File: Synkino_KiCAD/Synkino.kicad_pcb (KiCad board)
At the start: 2 copper layers, 88.4 x 82.3 mm, 180 parts, among them J1 Conn_01x02_Male, J10 EYE8_OUT, J11 EYE4_OUT, J12 2.5mm, J13 EYE5_OUT, J2 2.5mm, J3 3.5mm, J4 Micro_SD_Card_Det_Hirose_DM3AT, J5 EYE1_OUT, J6 EYE6_OUT, J7 EYE2_OUT, J8 EYE7_OUT, J9 EYE3_OUT, Q1 IRF7319, Q2 BC847, SW1 SW_Push, SW2 Rotary_Encoder_Switch, SW3 SW_Push, U1 MCP1702T-5002E/MB, U10 ATMEGA328P-AU, U11 QRE1113, U12 QRE1113, U13 QRE1113, U14 QRE1113, U15 QRE1113, U16 QRE1113, U18 QRE1113, U2 ATMEGA328P-AU, U3 74HC4050, U4 SPIOLED128x64, U5 AP7312-1833W6-7, U6 74HC14, U7 VS1053B, U8 MAX4741, U9 QRE1113, X1 FTDIconn, X2 ICSP, X3 FTDIconn, X4 ICSP, Y1 16Mhz, Y2 12.288MHz, Y3 16Mhz

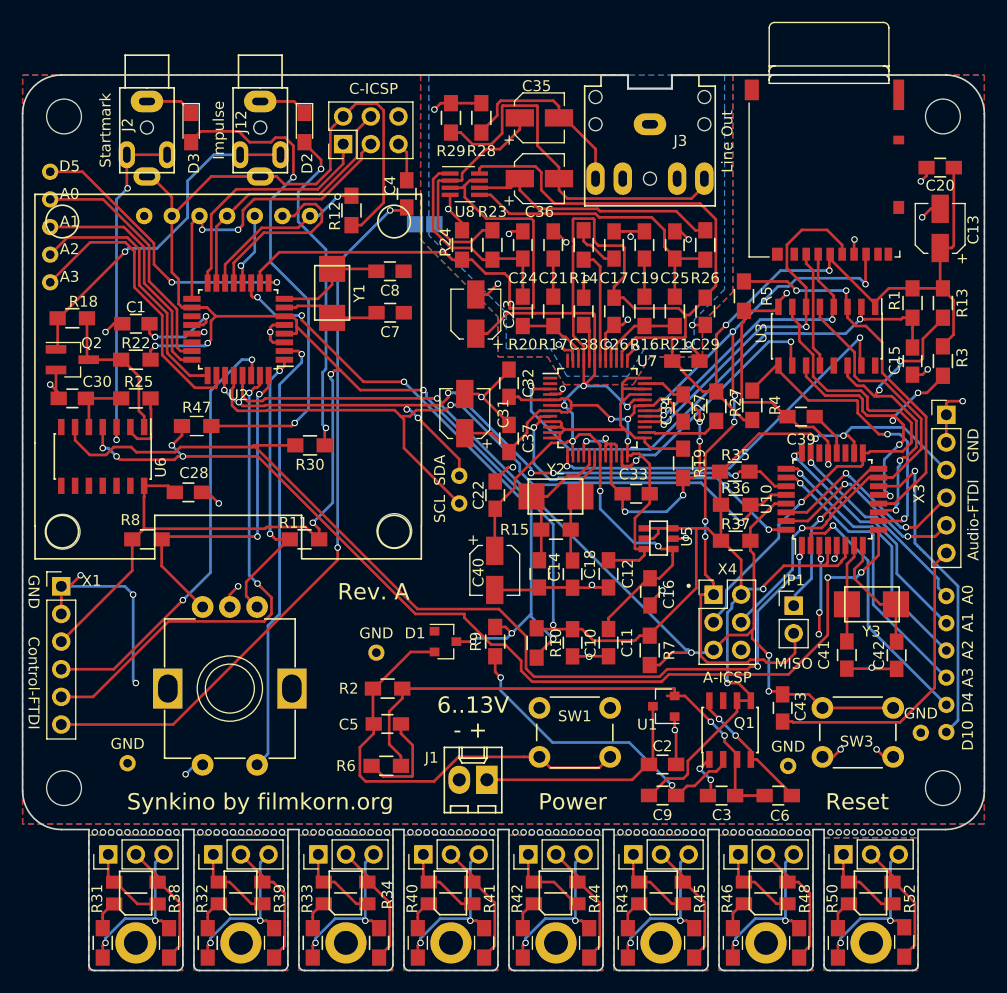
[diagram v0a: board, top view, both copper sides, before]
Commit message: Beautification
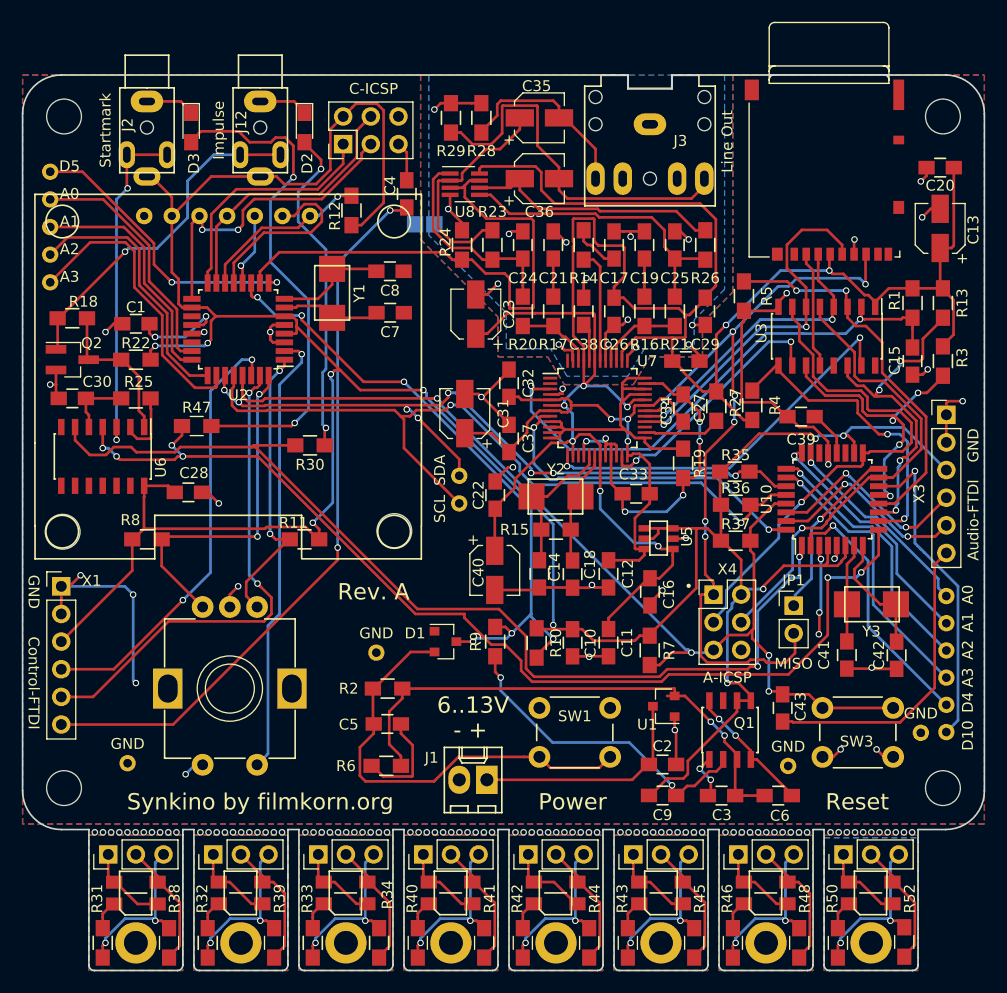
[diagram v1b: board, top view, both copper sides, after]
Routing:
- net GND: track 176.0 -> 174.2 mm
- net +5V: track 283.3 -> 282.3 mm
- net +3V3: track 220.5 -> 219.8 mm
